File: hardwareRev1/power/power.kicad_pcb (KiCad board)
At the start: 2 copper layers, 28 parts, among them IC1 ATTINY24A-M-FIXED, P1 VIN, P2 CONN_11X2, P3 AVRProg, U1 TPS63020, U2 NCP508

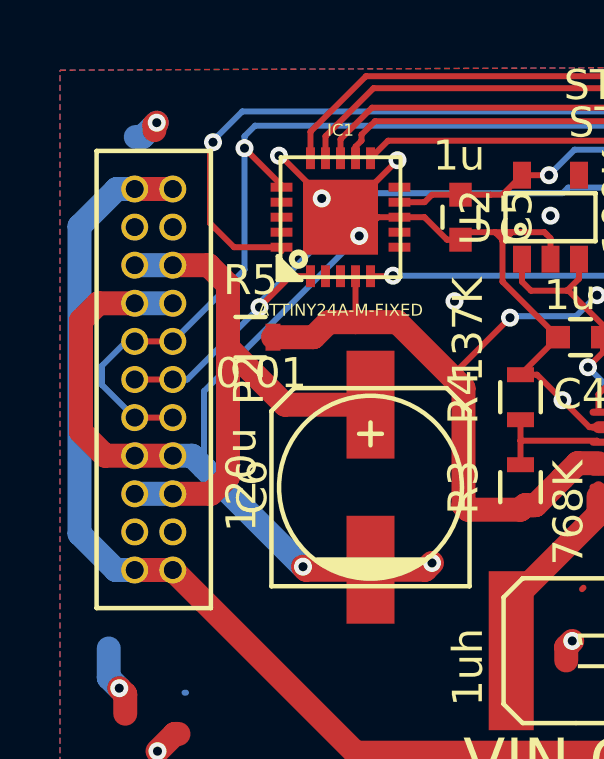
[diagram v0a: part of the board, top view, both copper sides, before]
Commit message: added the radio .
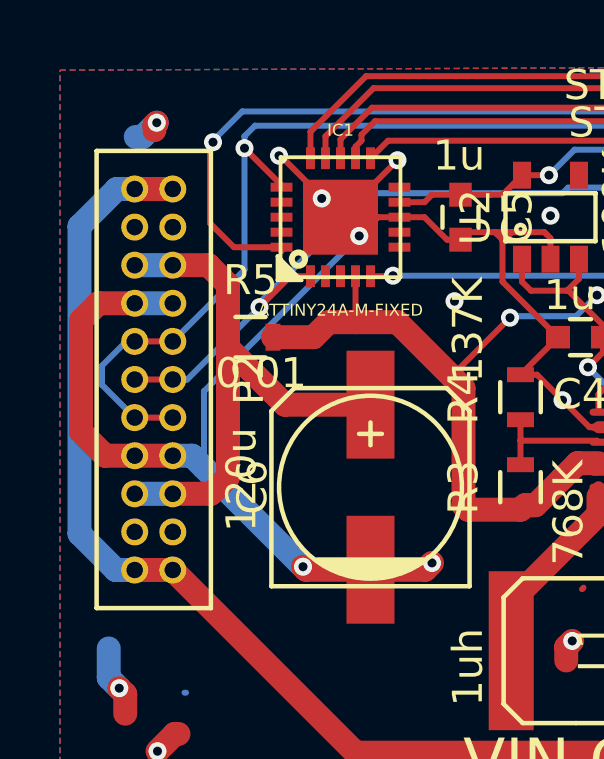
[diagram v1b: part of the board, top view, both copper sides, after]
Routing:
- net GND: track 127.2 -> 119.3 mm, vias 16 -> 9
- net (no net): track 0.51 -> 8.34 mm, vias 2 -> 9
